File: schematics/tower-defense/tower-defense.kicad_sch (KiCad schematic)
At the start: 6 parts, among them J1 Conn_01x28_Socket, J2 Conn_01x28_Socket, J3 Barrel_Jack_Switch, J4 Conn_01x16_Socket, J5 Conn_01x04_Socket, U1 COM-09032

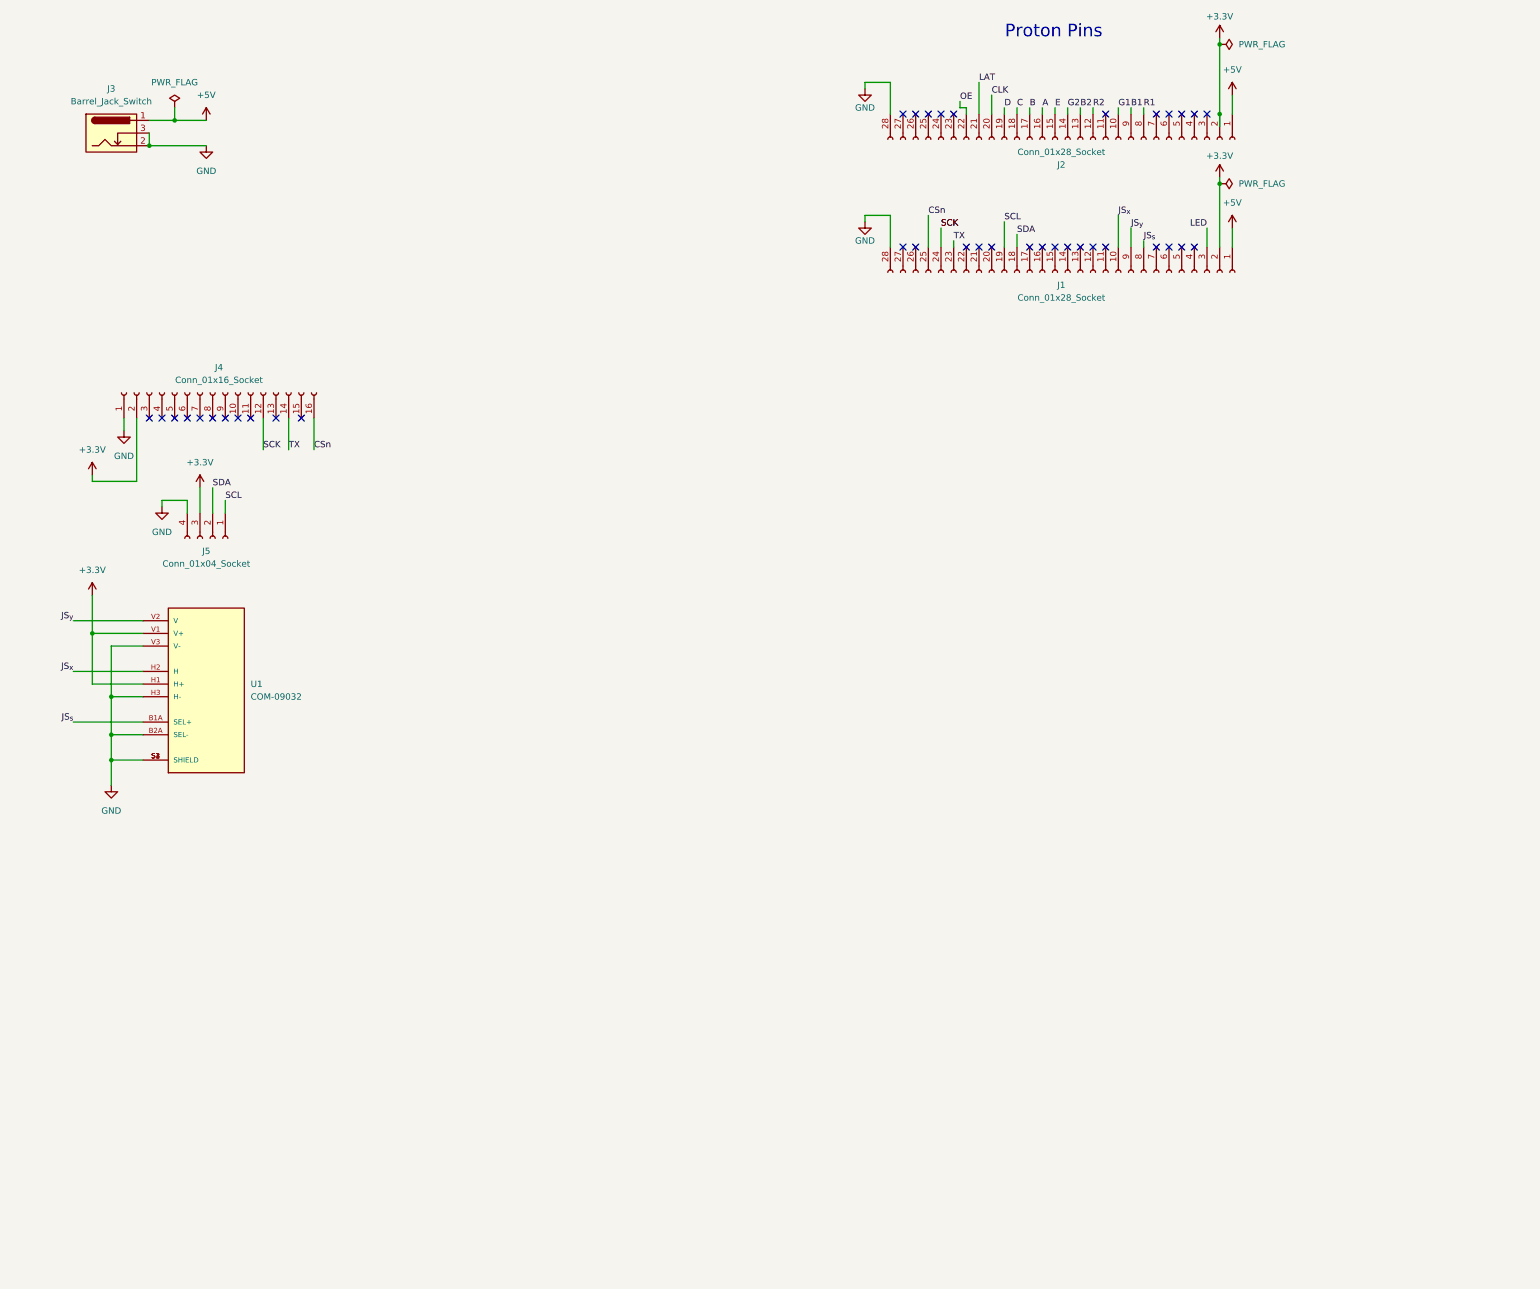
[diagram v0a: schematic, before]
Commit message: complete pcb v1
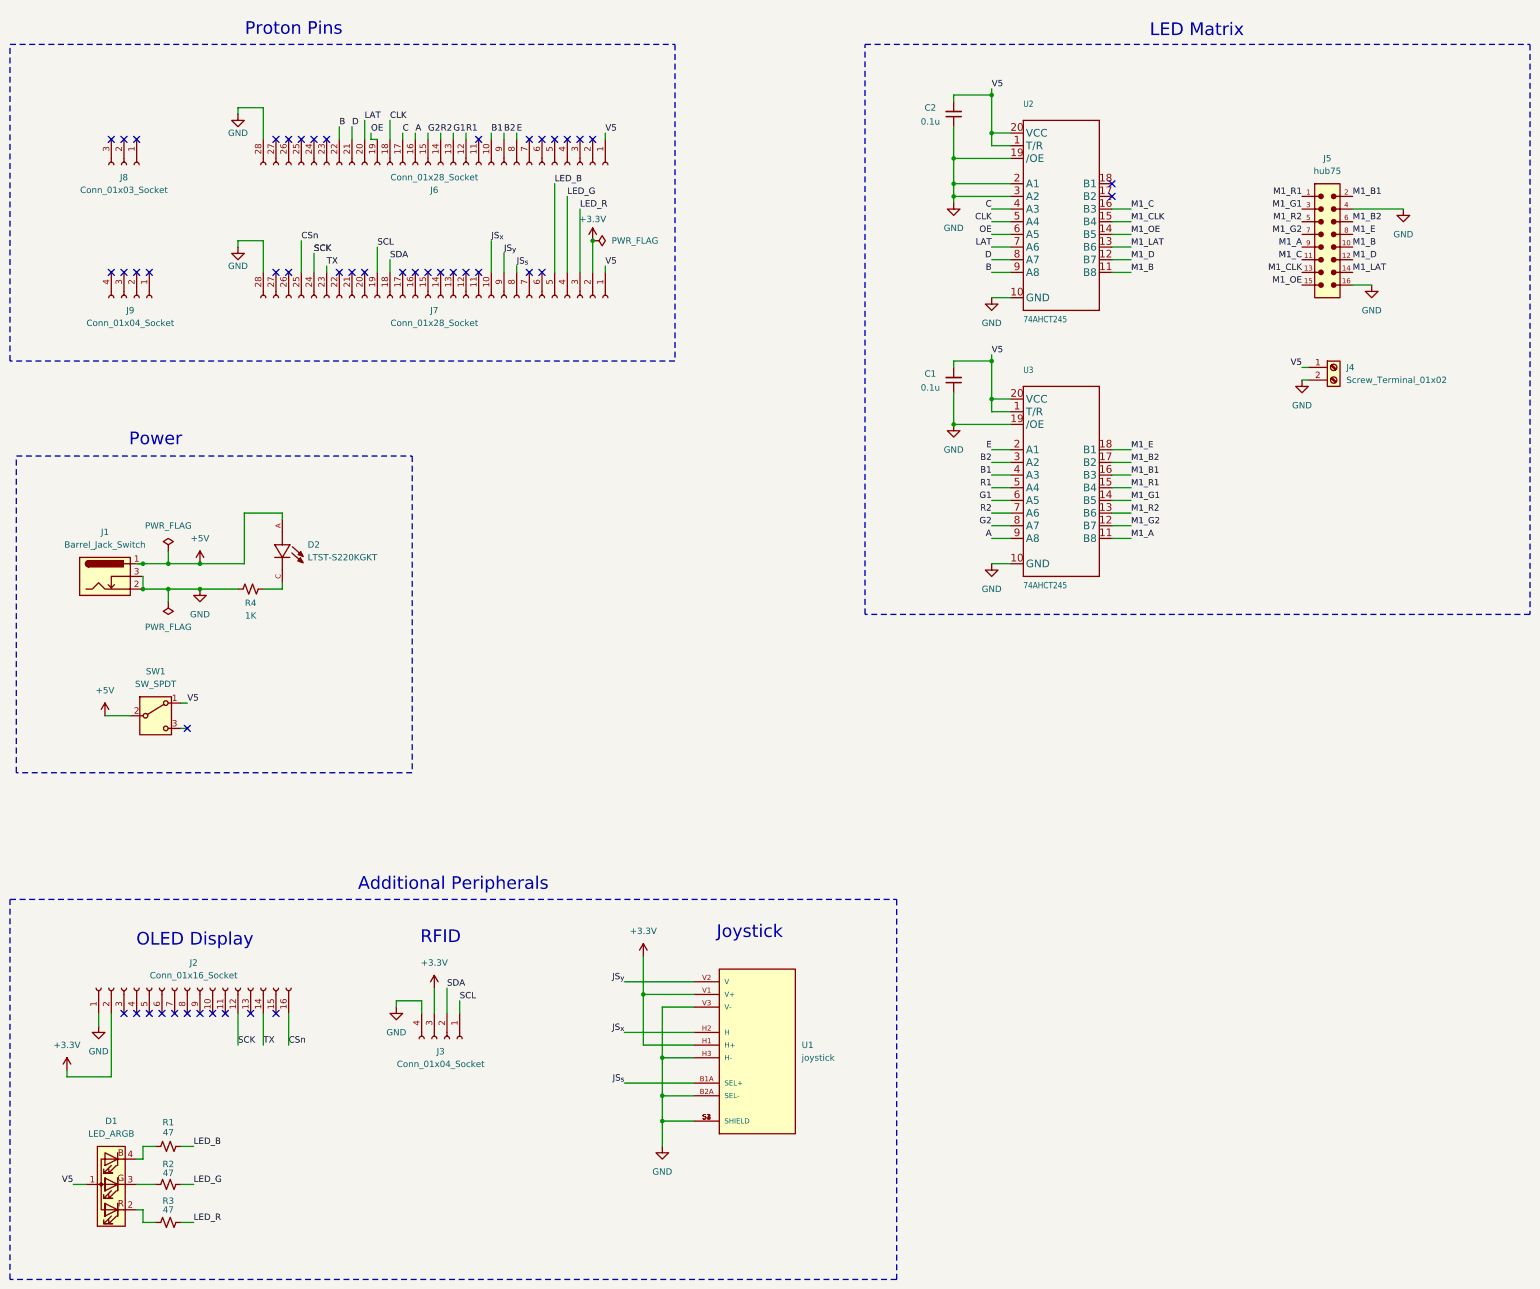
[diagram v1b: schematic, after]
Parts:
- removed U1: COM-09032, Tower_Defense:XDCR_COM-09032, symbol tower_defense:COM-09032
- added C1, C2: 0.1u, Capacitor_SMD:C_0603_1608Metric, symbol Device:C_Small
- added D1: LED_ARGB, Connector_PinSocket_2.54mm:PinSocket_1x04_P2.54mm_Vertical, symbol Device:LED_ARGB
- added D2: LTST-S220KGKT, Tower_Defense:status_led, symbol tower_defense:LTST-S220KGKT
- added J4: Screw_Terminal_01x02, Tower_Defense:screw-terminal, symbol Connector:Screw_Terminal_01x02
- added J5: hub75, Tower_Defense:hub75, symbol tower_defense:hub75
- added J8: Conn_01x03_Socket, Connector_PinSocket_2.54mm:PinSocket_1x03_P2.54mm_Vertical, symbol Connector:Conn_01x03_Socket
- added J9: Conn_01x04_Socket, Connector_PinSocket_2.54mm:PinSocket_1x04_P2.54mm_Vertical, symbol Connector:Conn_01x04_Socket
- added R1, R2, R3: 47, Resistor_SMD:R_0603_1608Metric, symbol Device:R_Small_US
- added R4: 1K, Resistor_SMD:R_0603_1608Metric, symbol Device:R_Small_US
- added SW1: SW_SPDT, Tower_Defense:power_switch, symbol Switch:SW_SPDT
- added U1: joystick, Tower_Defense:joystick, symbol tower_defense:joystick
- added U2, U3: 74AHCT245, Tower_Defense:74HTC245, symbol Adafruit RGB Matrix Bonnet-eagle-import:74LCX245
- renumbered J3 to J1, J4 to J2, J5 to J3, J2 to J6, J1 to J7
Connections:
- net +3.3V: now also U1.H1 (H+), U1.V1 (V+); no longer J6.2 (Pin_2)
- net +5V: now also D2.A, SW1.2 (B); no longer J6.1 (Pin_1), J7.1 (Pin_1)
- net A: now also U3.9 (A8)
- net B: now also J6.22 (Pin_22), U2.9 (A8); no longer J6.17 (Pin_17)
- net B1: now also J6.10 (Pin_10), U3.4 (A3); no longer J6.9 (Pin_9)
- net B2: now also J6.9 (Pin_9), U3.3 (A2); no longer J6.13 (Pin_13)
- net C: now also J6.17 (Pin_17), U2.4 (A3); no longer J6.18 (Pin_18)
- net CLK: now also J6.18 (Pin_18), U2.5 (A4); no longer J6.20 (Pin_20)
- net D: now also J6.21 (Pin_21), U2.8 (A7); no longer J6.19 (Pin_19)
- net E: now also J6.8 (Pin_8), U3.2 (A1); no longer J6.15 (Pin_15)
- net G1: now also J6.13 (Pin_13), U3.6 (A5); no longer J6.10 (Pin_10)
- net G2: now also J6.15 (Pin_15), U3.8 (A7); no longer J6.14 (Pin_14)
- net GND: now also C1.1, C2.1, J4.2 (Pin_2), J5.16, J5.4, R4.1, U1.B2A (SEL-), U1.H3 (H-), U1.S1 (SHIELD), U1.S2 (SHIELD), U1.S3 (SHIELD), U1.S4 (SHIELD), U1.V3 (V-), U2.10 (GND), U2.19 (/OE), U2.2 (A1), U2.3 (A2), U3.10 (GND), U3.19 (/OE)
- net JS_{s}: now also U1.B1A (SEL+)
- net JS_{x}: now also U1.H2 (H)
- net JS_{y}: now also U1.V2 (V)
- net LAT: now also J6.20 (Pin_20), U2.7 (A6); no longer J6.21 (Pin_21)
- net OE: now also J6.19 (Pin_19), U2.6 (A5); no longer J6.22 (Pin_22)
- net R1: now also J6.12 (Pin_12), U3.5 (A4); no longer J6.8 (Pin_8)
- net R2: now also J6.14 (Pin_14), U3.7 (A6); no longer J6.12 (Pin_12)
- net LED_G: now reaches J7.4 (Pin_4)
- net LED_G: now also R2.2
- net LED_B: now reaches J7.5 (Pin_5)
- net LED_B: now also R1.2
- net LED renamed LED_R
- net LED_R: now also R3.2
- new net: D1.4 (BK), R1.1
- new net: D2.C, R4.2
- new net: D1.3 (GK), R2.1
- new net: D1.2 (RK), R3.1
- new net M1_A: J5.9, U3.11 (B8)
- new net M1_B: J5.10, U2.11 (B8)
- new net M1_B1: J5.2, U3.16 (B3)
- new net M1_B2: J5.6, U3.17 (B2)
- new net M1_C: J5.11, U2.16 (B3)
- new net M1_CLK: J5.13, U2.15 (B4)
- new net M1_D: J5.12, U2.12 (B7)
- new net M1_E: J5.8, U3.18 (B1)
- new net M1_G1: J5.3, U3.14 (B5)
- new net M1_G2: J5.7, U3.12 (B7)
- new net M1_LAT: J5.14, U2.13 (B6)
- new net M1_OE: J5.15, U2.14 (B5)
- new net M1_R1: J5.1, U3.15 (B4)
- new net M1_R2: J5.5, U3.13 (B6)
- new net V5: C1.2, C2.2, D1.1 (A), J4.1 (Pin_1), J6.1 (Pin_1), J7.1 (Pin_1), SW1.1 (A), U2.1 (T/R), U2.20 (VCC), U3.1 (T/R), U3.20 (VCC)
- no-connect marks 38 -> 47
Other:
- note added: "Additional Peripherals"
- note added: "Joystick"
- note added: "LED Matrix"
- note added: "OLED Display"
- note added: "Power"
- note added: "RFID"
- moved on the sheet: J1, J2, J3, J6, J7
